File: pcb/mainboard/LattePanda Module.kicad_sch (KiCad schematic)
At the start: 15 parts, among them J1 Conn_01x03_Pin, J84 Conn_01x02_Pin

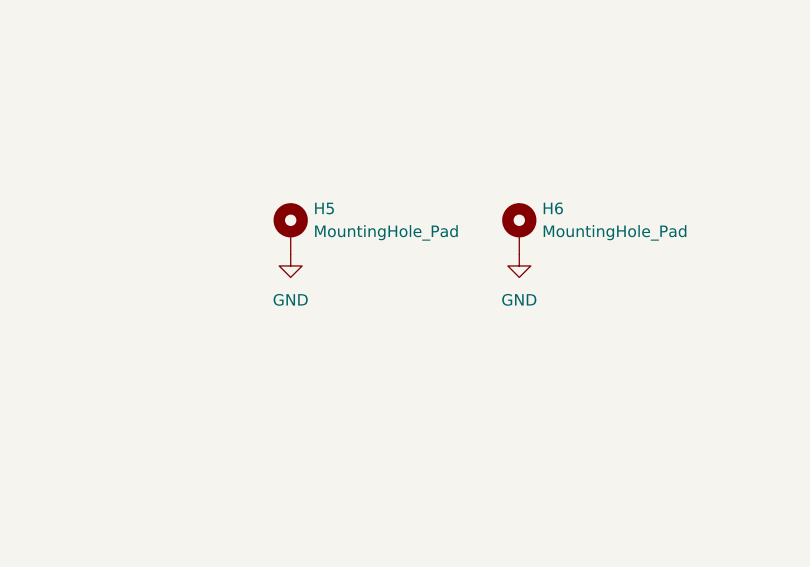
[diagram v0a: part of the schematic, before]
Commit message: before i aply ungrounding changes to moutning holes
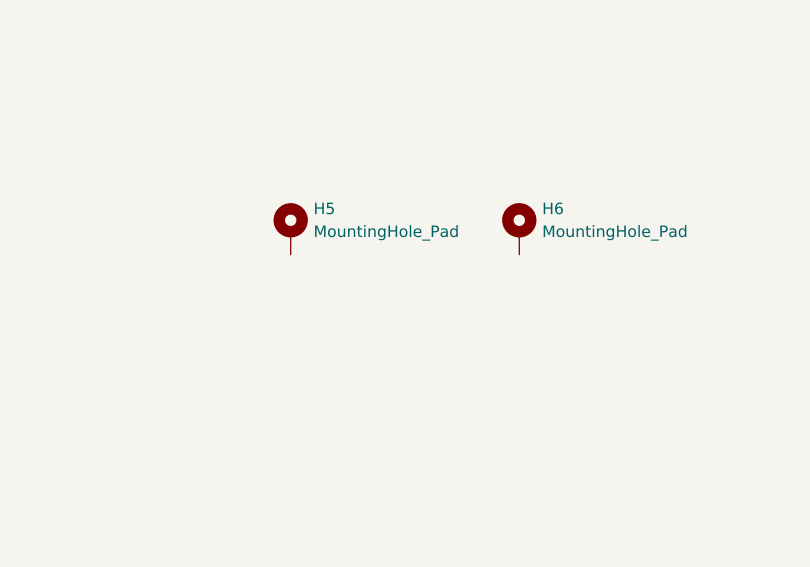
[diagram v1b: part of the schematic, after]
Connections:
- net GND: no longer H5.1, H6.1
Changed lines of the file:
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@@
-	)
-	(symbol
-		(lib_id "power:GND")
-		(at 439.42 302.26 0)
-		(unit 1)
-		(exclude_from_sim no)
-		(in_bom yes)
-		(on_board yes)
-		(dnp no)
-		(fields_autoplaced yes)
-		(property "Reference" "#PWR012"
-			(at 439.42 308.61 0)
-			(effects
-				(font
-					(size 1.27 1.27)
-				)
-				(hide yes)
-			)
-		)
-		(property "Value" "GND"
-			(at 439.42 307.34 0)
-			(effects
-				(font
-					(size 1.27 1.27)
-				)
-			)
-		)
-		(property "Footprint" ""
-			(at 439.42 302.26 0)
-			(effects
-				(font
-					(size 1.27 1.27)
-				)
-				(hide yes)
-			)
-		)
-		(property "Datasheet" ""
-			(at 439.42 302.26 0)
-			(effects
-				(font
-					(size 1.27 1.27)
-				)
-				(hide yes)
-			)
-		)
-		(property "Description" ""
-			(at 439.42 302.26 0)
-			(effects
-				(font
-					(size 1.27 1.27)
-				)
-				(hide yes)
-			)
-		)
-		(pin "1"
-		)
-		(instances
-			(project "[DFR1142]Lite Carrier for LattePanda Mu"
-				(path "/2a6d114a-7fd7-4207-b5f7-4ea9c34f36aa/6eee02c2-78c9-4e83-9ccf-e0f7690b57bf"
-					(reference "#PWR012")
-					(unit 1)
-				)
-			)
-		)
 	)
 	(symbol
@@
 					(unit 1)
 				)
-			)
-		)
-	)
-	(symbol
-		(lib_id "power:GND")
-		(at 414.02 302.26 0)
-		(unit 1)
-		(exclude_from_sim no)
-		(in_bom yes)
-		(on_board yes)
-		(dnp no)
-		(fields_autoplaced yes)
-		(property "Reference" "#PWR011"
-			(at 414.02 308.61 0)
-			(effects
-				(font
-					(size 1.27 1.27)
-				)
-				(hide yes)
-			)
-		)
-		(property "Value" "GND"
-			(at 414.02 307.34 0)
-			(effects
-				(font
-					(size 1.27 1.27)
-				)
-			)
-		)
-		(property "Footprint" ""
-			(at 414.02 302.26 0)
-			(effects
-				(font
-					(size 1.27 1.27)
-				)
-				(hide yes)
-			)
-		)
-		(property "Datasheet" ""
-			(at 414.02 302.26 0)
-			(effects
-				(font
-					(size 1.27 1.27)
-				)
-				(hide yes)
-			)
-		)
-		(property "Description" ""
-			(at 414.02 302.26 0)
-			(effects
-				(font
-					(size 1.27 1.27)
-				)
-				(hide yes)
-			)
-		)
-		(pin "1"
-		)
-		(instances
-			(project "[DFR1142]Lite Carrier for LattePanda Mu"
-				(path "/2a6d114a-7fd7-4207-b5f7-4ea9c34f36aa/6eee02c2-78c9-4e83-9ccf-e0f7690b57bf"
-					(reference "#PWR011")
-					(unit 1)
-				)

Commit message: a
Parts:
- H78, H79, H80: now in the parts list
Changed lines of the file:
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@@
 		(unit 1)
 		(exclude_from_sim no)
-		(in_bom no)
+		(in_bom yes)
 		(on_board yes)
 		(dnp no)
@@
 		(unit 1)
 		(exclude_from_sim no)
-		(in_bom no)
+		(in_bom yes)
 		(on_board yes)
 		(dnp no)
@@
 		(unit 1)
 		(exclude_from_sim no)
-		(in_bom no)
-		(on_board yes)
-		(dnp no)
+		(in_bom yes)
+		(on_board yes)
+		(dnp no)
